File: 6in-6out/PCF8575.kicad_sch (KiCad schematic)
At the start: 16 parts, among them U13 PCF8575DBR, U14 PCF8575DBR

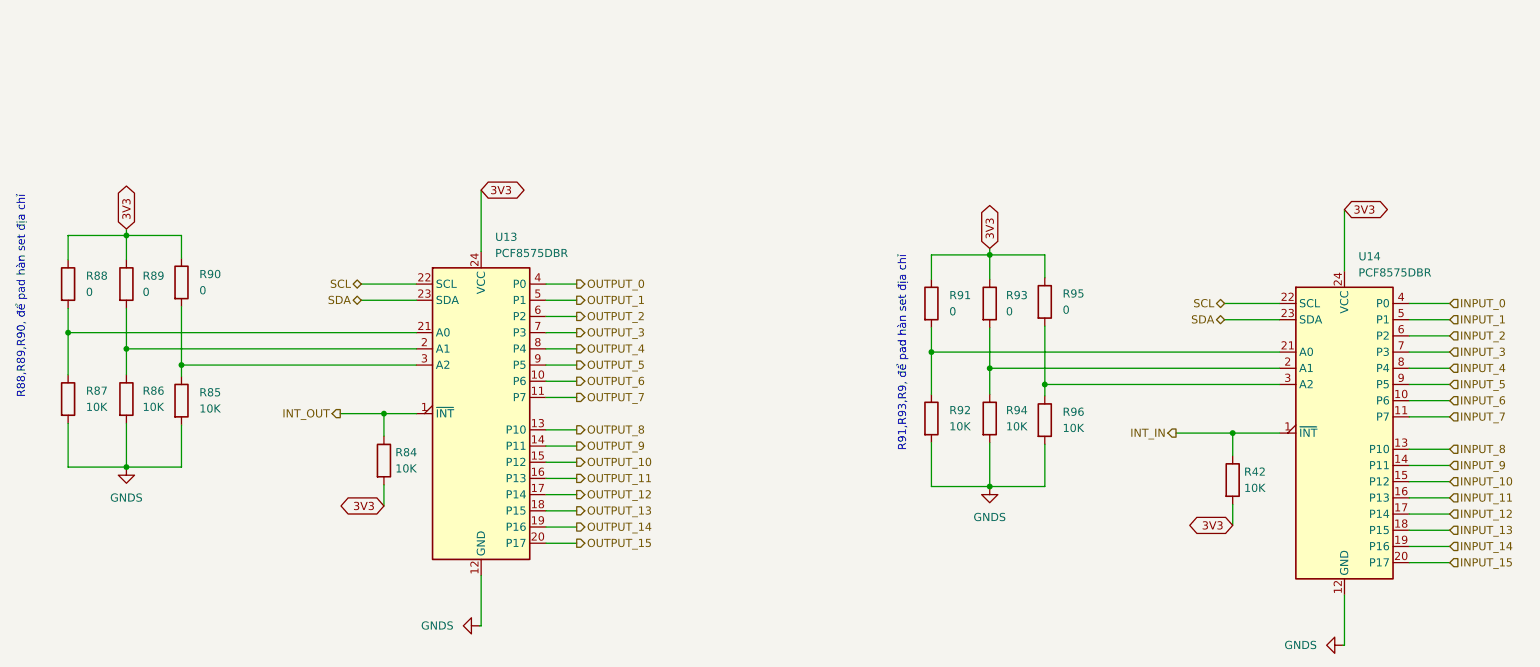
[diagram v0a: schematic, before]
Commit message: no message
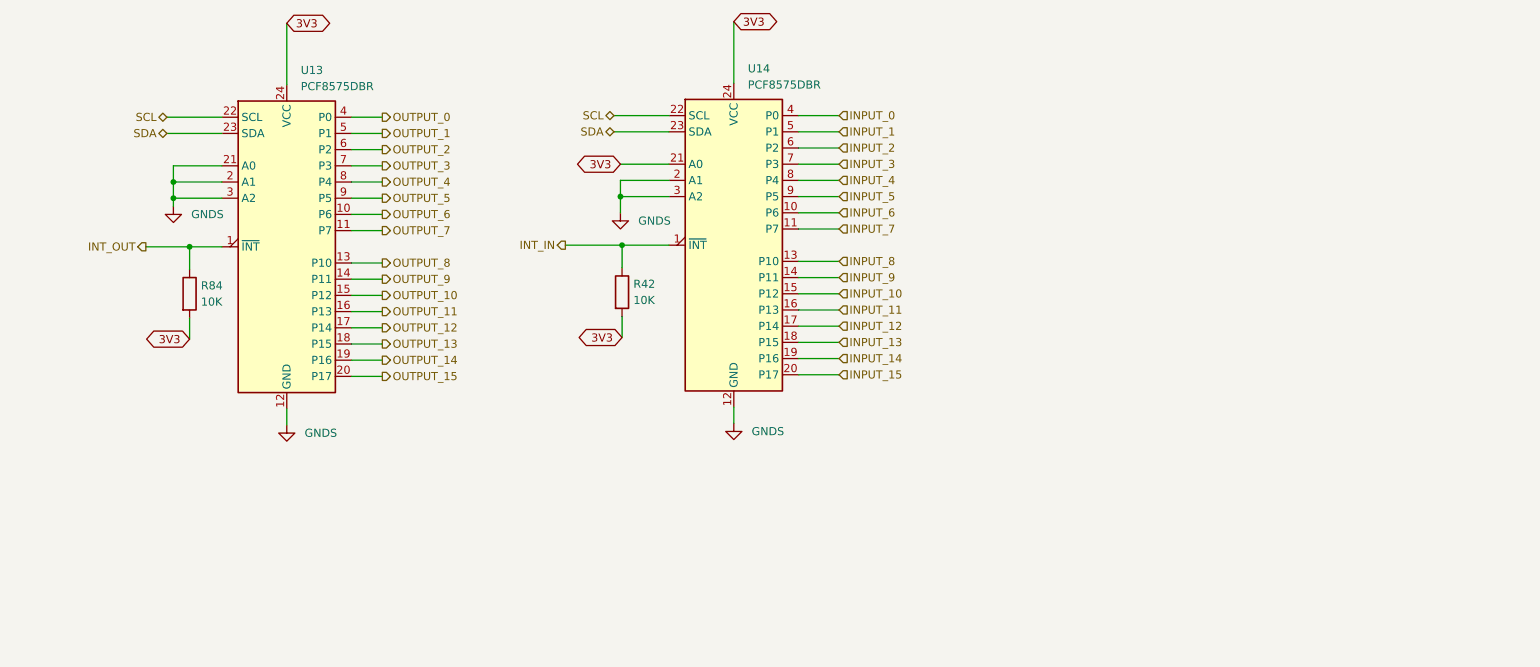
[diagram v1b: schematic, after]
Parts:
- removed R85, R86, R87, R92, R94, R96: 10K, Resistor_SMD:R_0603_1608Metric_Pad0.98x0.95mm_HandSolder, symbol Device:R
- removed R88, R89, R90, R91, R93, R95: 0, Resistor_SMD:R_0603_1608Metric_Pad0.98x0.95mm_HandSolder, symbol Device:R
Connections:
- net 3V3: now also U14.21 (A0)
- net GNDS: now also U13.2 (A1), U13.21 (A0), U13.3 (A2), U14.2 (A1), U14.3 (A2)
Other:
- note removed: "R88,R89,R90, để pad hàn set địa chỉ"
- note removed: "R91,R93,R9, để pad hàn set địa chỉ"
- moved on the sheet: R42, R84, U13, U14
